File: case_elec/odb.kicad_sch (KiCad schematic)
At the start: 9 parts

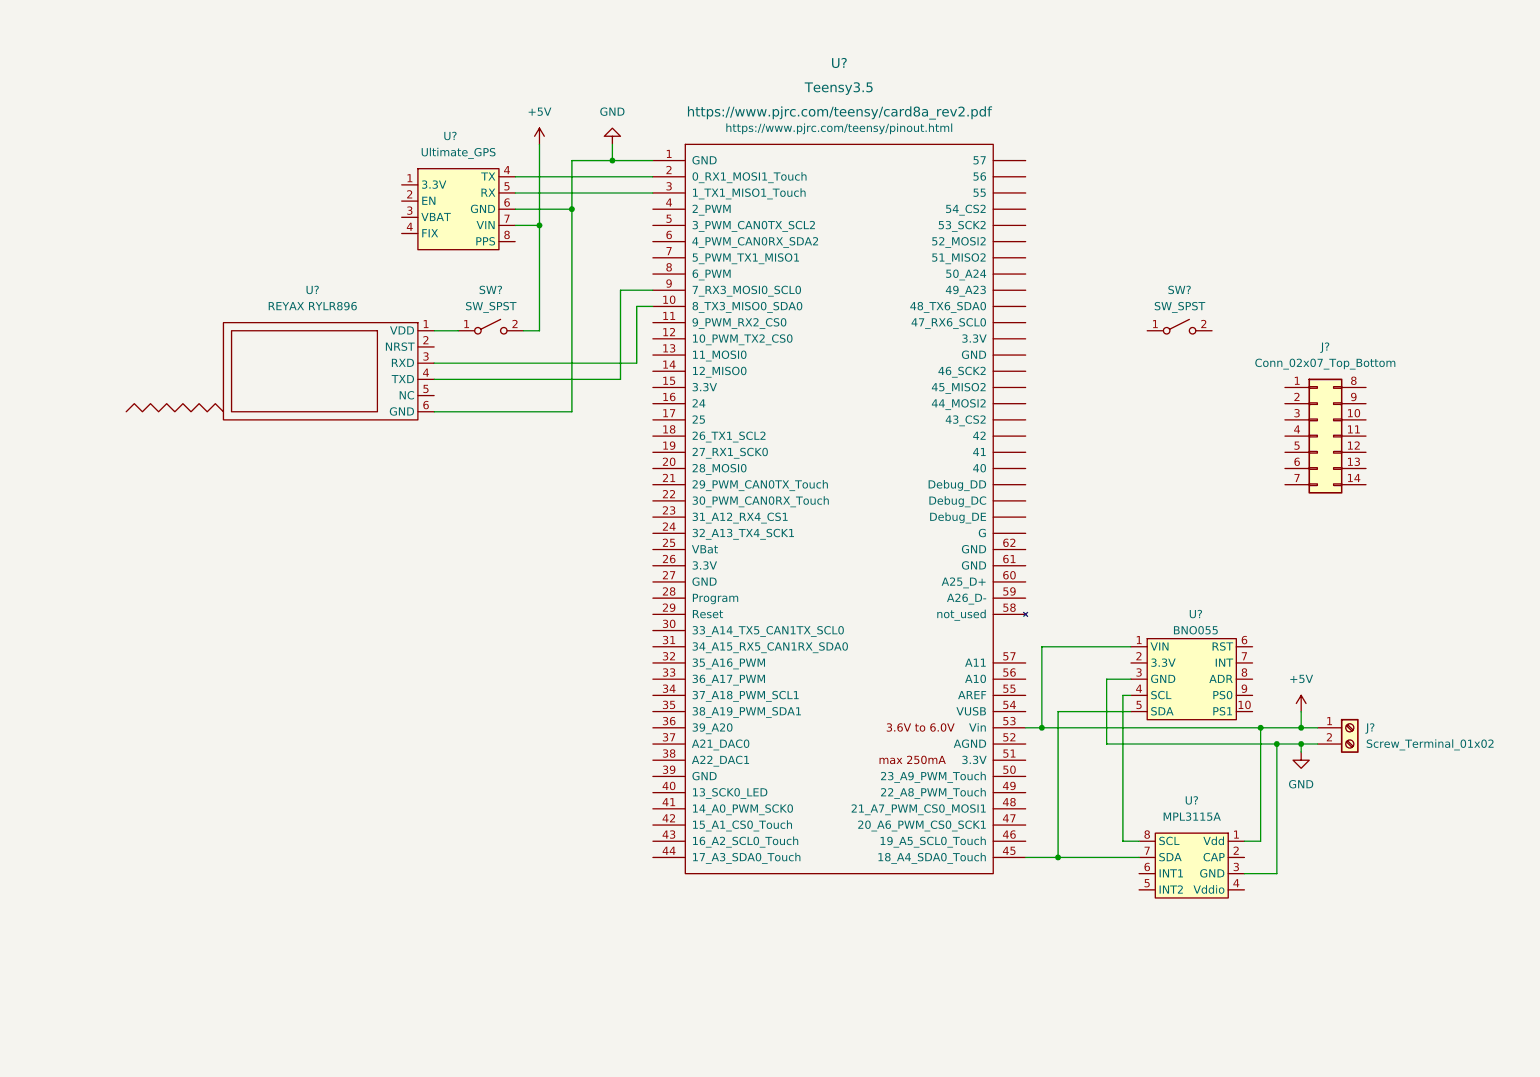
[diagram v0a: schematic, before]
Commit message: complétion du schéma électrique
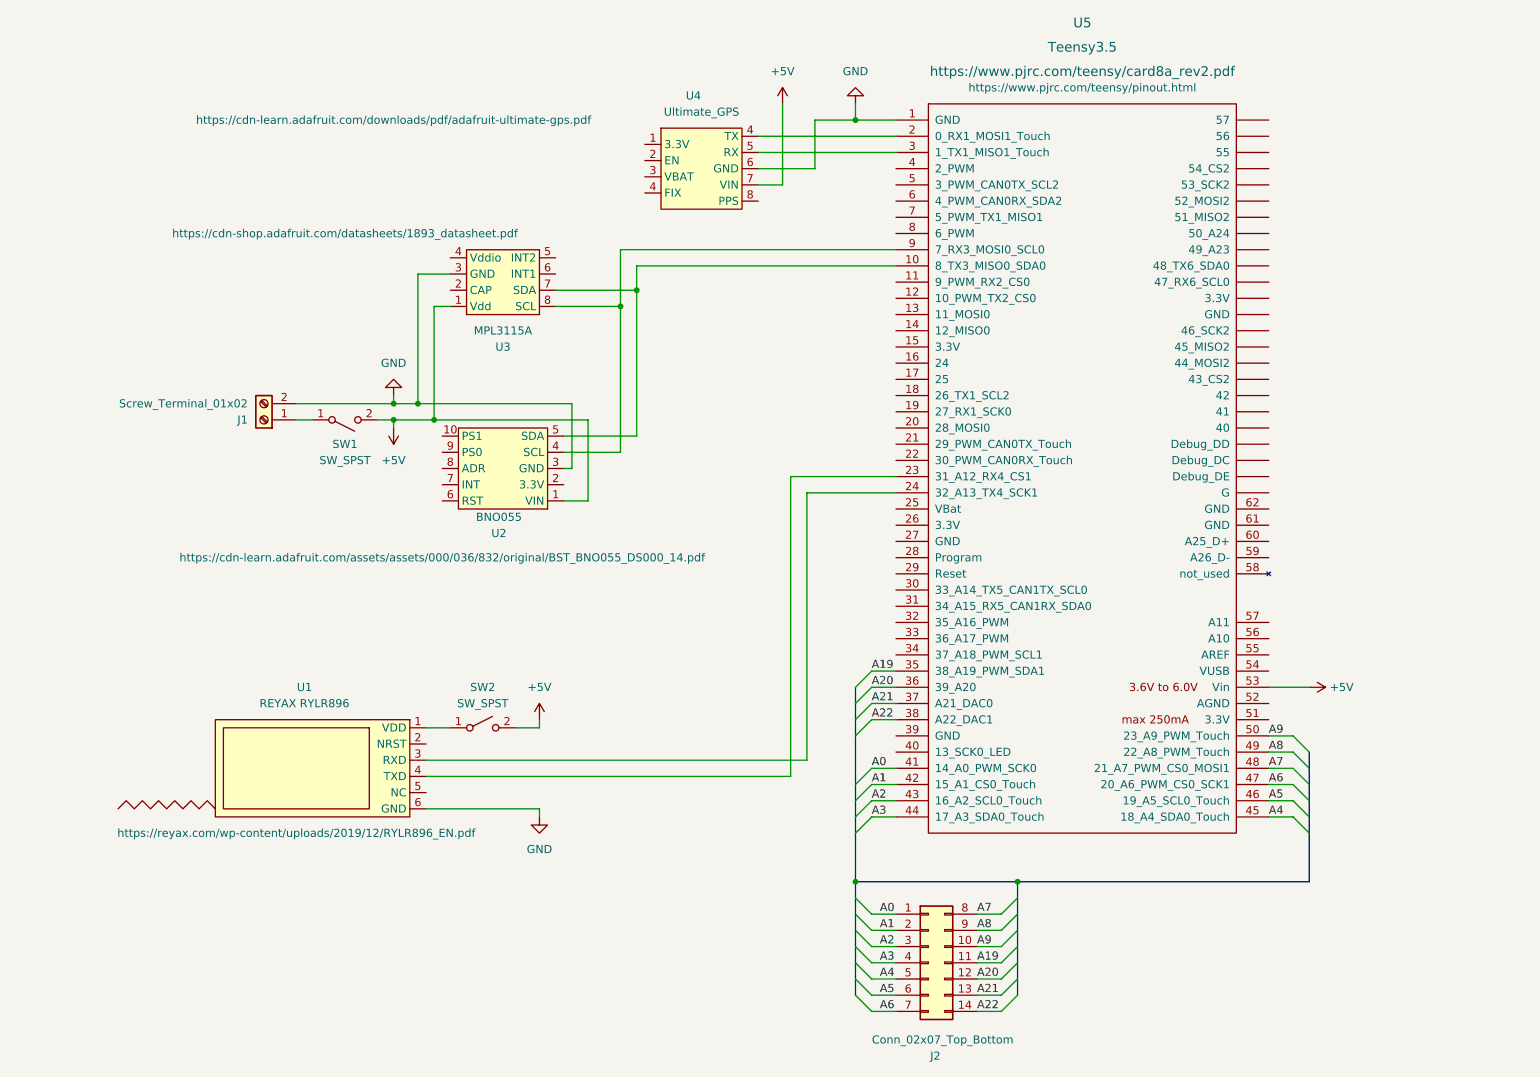
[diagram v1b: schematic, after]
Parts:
- removed J?: Screw_Terminal_01x02, symbol Connector:Screw_Terminal_01x02
- removed SW?: SW_SPST, symbol Switch:SW_SPST
- removed U?: MPL3115A, symbol Adafruit_sensors:MPL3115A
- removed U?: BNO055, symbol Adafruit_sensors:BNO055
- added J1: Screw_Terminal_01x02, symbol Connector:Screw_Terminal_01x02
- added SW1: SW_SPST, symbol Switch:SW_SPST
- added U2: BNO055, symbol Adafruit_sensors:BNO055
- added U3: MPL3115A, symbol Adafruit_sensors:MPL3115A
- U1: renamed from U?; Command (none) -> https://reyax.com/wp-content/uploads/2019/12/LoRa-AT-Comman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
- gave numbers to parts that had none: 4
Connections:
- net +5V: now also SW1.2 (B), U2.1 (VIN), U3.1 (Vdd)
- net GND: now also J1.2 (Pin_2), U2.3 (GND), U3.3 (GND)
- net A4: now reaches U5.45 (18_A4_SDA0_Touch)
- net A4: now also J2.5 (Pin_5)
- net A0: now reaches J2.1 (Pin_1)
- net A0: now also U5.41 (14_A0_PWM_SCK0)
- net A9: now reaches J2.10 (Pin_10)
- net A9: now also U5.50 (23_A9_PWM_Touch)
- net A19: now reaches J2.11 (Pin_11)
- net A19: now also U5.35 (38_A19_PWM_SDA1)
- net A20: now reaches J2.12 (Pin_12)
- net A20: now also U5.36 (39_A20)
- net A21: now reaches J2.13 (Pin_13)
- net A21: now also U5.37 (A21_DAC0)
- net A22: now reaches J2.14 (Pin_14)
- net A22: now also U5.38 (A22_DAC1)
- net A1: now reaches J2.2 (Pin_2)
- net A1: now also U5.42 (15_A1_CS0_Touch)
- net A2: now reaches J2.3 (Pin_3)
- net A2: now also U5.43 (16_A2_SCL0_Touch)
- net A3: now reaches J2.4 (Pin_4)
- net A3: now also U5.44 (17_A3_SDA0_Touch)
- net A5: now reaches J2.6 (Pin_6)
- net A5: now also U5.46 (19_A5_SCL0_Touch)
- net A6: now reaches J2.7 (Pin_7)
- net A6: now also U5.47 (20_A6_PWM_CS0_SCK1)
- net A7: now reaches J2.8 (Pin_8)
- net A7: now also U5.48 (21_A7_PWM_CS0_MOSI1)
- net A8: now reaches J2.9 (Pin_9)
- net A8: now also U5.49 (22_A8_PWM_Touch)
- net at U5.10 (8_TX3_MISO0_SDA0): now also U2.5 (SDA), U3.7 (SDA); no longer U1.3 (RXD)
- net at U5.23 (31_A12_RX4_CS1): now also U1.4 (TXD)
- net at U5.24 (32_A13_TX4_SCK1): now also U1.3 (RXD)
- net at U5.9 (7_RX3_MOSI0_SCL0): now also U2.4 (SCL), U3.8 (SCL); no longer U1.4 (TXD)
- new net: J1.1 (Pin_1), SW1.1 (A)
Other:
- moved on the sheet: J2, SW2, U4, U5

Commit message: Mise à jour du pcb
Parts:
- J2: footprint (none) -> Connector_Molex:Molex_Nano-Fit_105310-xx14_2x07_P2.50mm_Vertical
- SW2: footprint (none) -> common_misc:SW
- U1: footprint (none) -> Reyax:RYLR896
- U2: footprint (none) -> Adafruit_sensors:BNO055
- U3: footprint (none) -> Adafruit_sensors:MPL3115A2
- U4: footprint (none) -> Adafruit_sensors:Ultimate_GPS
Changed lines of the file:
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@@
       (effects (font (size 1.27 1.27)) (justify right))
     )
-    (property "Footprint" "" (id 2) (at 156.21 166.37 0)
+    (property "Footprint" "Connector_Molex:Molex_Nano-Fit_105310-xx14_2x07_P2.50mm_Vertical" (id 2) (at 156.21 166.37 0)
       (effects (font (size 1.27 1.27)) hide)
     )
@@
     (property "Reference" "U2" (id 0) (at 88.9 99.06 0))
     (property "Value" "BNO055" (id 1) (at 88.9 96.52 0))
-    (property "Footprint" "" (id 2) (at 96.52 93.98 0)
+    (property "Footprint" "Adafruit_sensors:BNO055" (id 2) (at 96.52 93.98 0)
       (effects (font (size 1.27 1.27)) hide)
     )
@@
     (property "Reference" "U4" (id 0) (at 119.38 30.48 0))
     (property "Value" "Ultimate_GPS" (id 1) (at 120.65 33.02 0))
-    (property "Footprint" "" (id 2) (at 113.665 35.56 0)
+    (property "Footprint" "Adafruit_sensors:Ultimate_GPS" (id 2) (at 113.665 35.56 0)
       (effects (font (size 1.27 1.27)) hide)
     )
@@
     (property "Reference" "U1" (id 0) (at 58.42 123.19 0))
     (property "Value" "REYAX RYLR896" (id 1) (at 58.42 125.73 0))
-    (property "Footprint" "" (id 2) (at 59.69 123.19 0)
+    (property "Footprint" "Reyax:RYLR896" (id 2) (at 59.69 123.19 0)
       (effects (font (size 1.27 1.27)) hide)
     )
@@
     (property "Reference" "SW2" (id 0) (at 86.36 123.19 0))
     (property "Value" "SW_SPST" (id 1) (at 86.36 125.73 0))
-    (property "Footprint" "" (id 2) (at 86.36 129.54 0)
+    (property "Footprint" "common_misc:SW" (id 2) (at 86.36 129.54 0)
       (effects (font (size 1.27 1.27)) hide)
     )
@@
     (property "Reference" "U3" (id 0) (at 89.535 69.85 0))
     (property "Value" "MPL3115A" (id 1) (at 89.535 67.31 0))
-    (property "Footprint" "" (id 2) (at 97.79 59.69 0)
+    (property "Footprint" "Adafruit_sensors:MPL3115A2" (id 2) (at 97.79 59.69 0)
       (effects (font (size 1.27 1.27)) hide)
     )
@@
     )
     (path "/55cf5624-44da-424d-9e40-f56e6ab73601"
-      (reference "J2") (unit 1) (value "Conn_02x07_Top_Bottom") (footprint "")
+      (reference "J2") (unit 1) (value "Conn_02x07_Top_Bottom") (footprint "Connector_Molex:Molex_Nano-Fit_105310-xx14_2x07_P2.50mm_Vertical")
     )
     (path "/9077b56f-c102-47b4-9a60-c432e96c7e85"
@@
     )
     (path "/c068de85-ccf9-478f-b6ba-b78ea8eb0dbf"
-      (reference "SW2") (unit 1) (value "SW_SPST") (footprint "")
+      (reference "SW2") (unit 1) (value "SW_SPST") (footprint "common_misc:SW")
     )
     (path "/9723626b-2488-483d-ac8f-0c4da911e062"
-      (reference "U1") (unit 1) (value "REYAX RYLR896") (footprint "")
+      (reference "U1") (unit 1) (value "REYAX RYLR896") (footprint "Reyax:RYLR896")
     )
     (path "/595afb03-5142-4518-8068-322873960ff6"
-      (reference "U2") (unit 1) (value "BNO055") (footprint "")
+      (reference "U2") (unit 1) (value "BNO055") (footprint "Adafruit_sensors:BNO055")
     )
     (path "/dce04994-4869-4e0d-8e66-d9270f6eb7e1"
-      (reference "U3") (unit 1) (value "MPL3115A") (footprint "")
+      (reference "U3") (unit 1) (value "MPL3115A") (footprint "Adafruit_sensors:MPL3115A2")
     )
     (path "/857fdb2b-599c-415c-9c78-a5968f20db3d"
-      (reference "U4") (unit 1) (value "Ultimate_GPS") (footprint "")
+      (reference "U4") (unit 1) (value "Ultimate_GPS") (footprint "Adafruit_sensors:Ultimate_GPS")
     )
     (path "/6dbf9b0b-d170-42c2-945f-d4ad0c4354aa"
